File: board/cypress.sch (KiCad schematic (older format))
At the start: 59 parts, among them J1 USB_MICRO_B, U1 CY7C68013A, U2 M25P16, X1 CRYSTAL

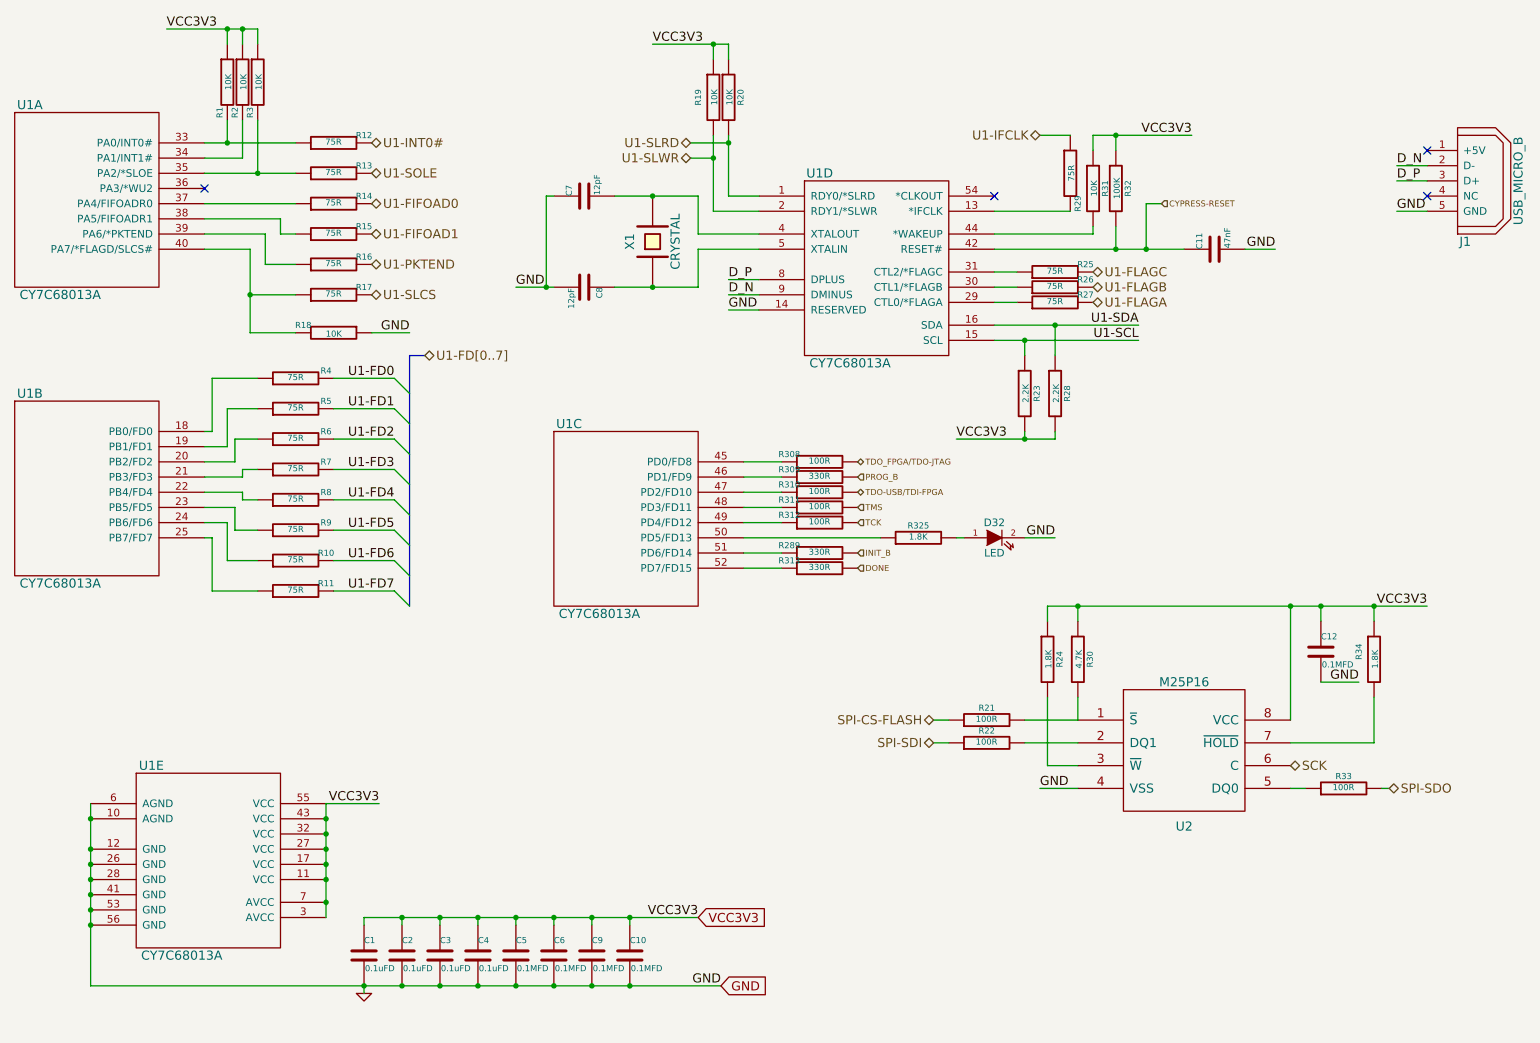
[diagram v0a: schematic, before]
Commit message: Issue #993
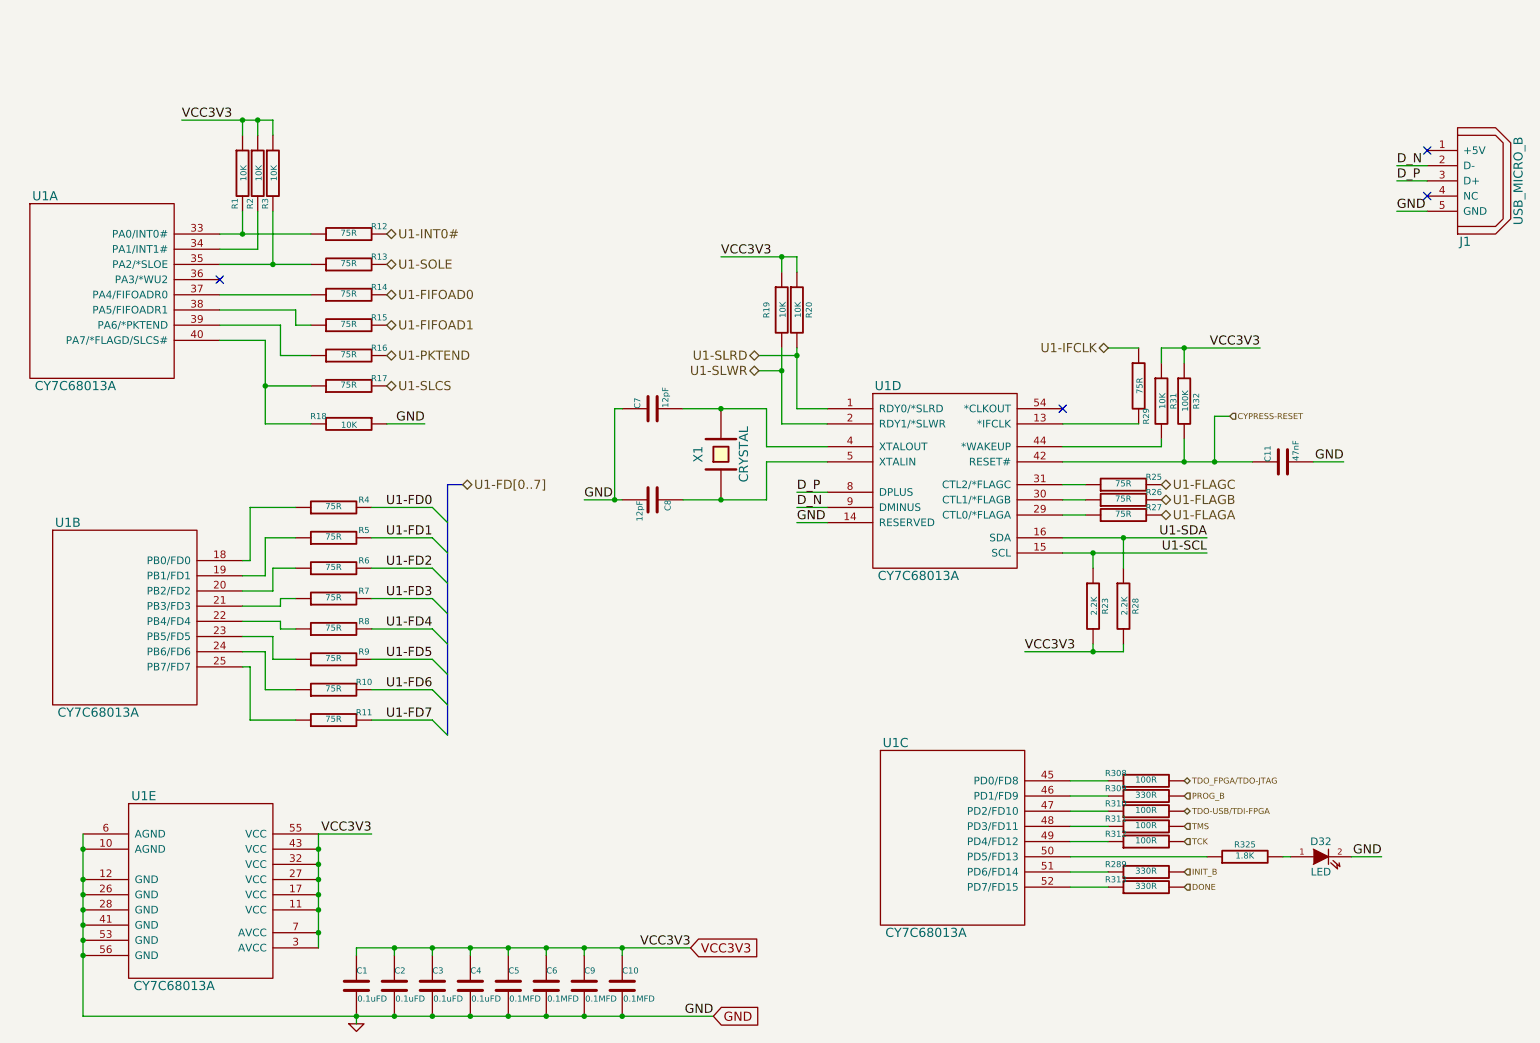
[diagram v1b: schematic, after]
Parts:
- removed C12: 0.1MFD, ~, symbol C
- removed R21, R22, R33: 100R, ~, symbol R
- removed R24, R34: 1.8K, ~, symbol R
- removed R30: 4.7K, ~, symbol R
- removed U2: M25P16, symbol M25P16
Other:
- moved on the sheet: C1, C10, C11, C2, C3, C4, C5, C6, C7, C8, C9, D32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
